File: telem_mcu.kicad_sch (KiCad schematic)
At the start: 28 parts, among them J3 Conn_01x06, J5 Micro_SD_Card, SW2 SW_Push, U3 STM32F373CCTx, X1 32.768kHz

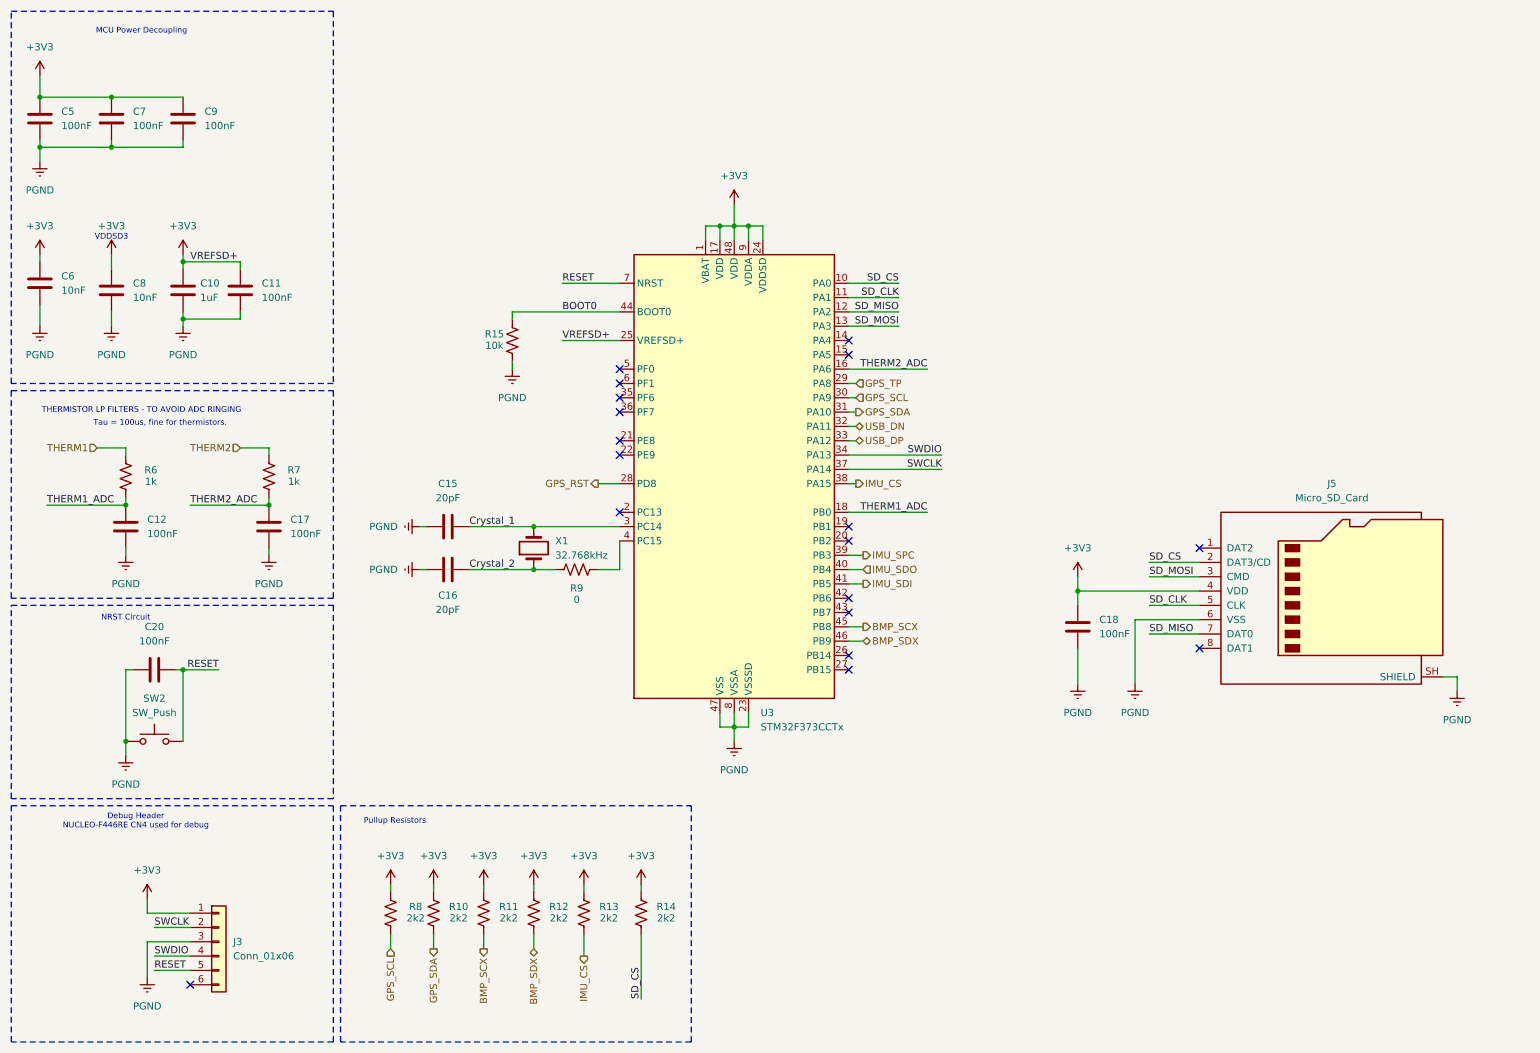
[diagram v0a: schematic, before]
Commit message: Updated schematics for rev2
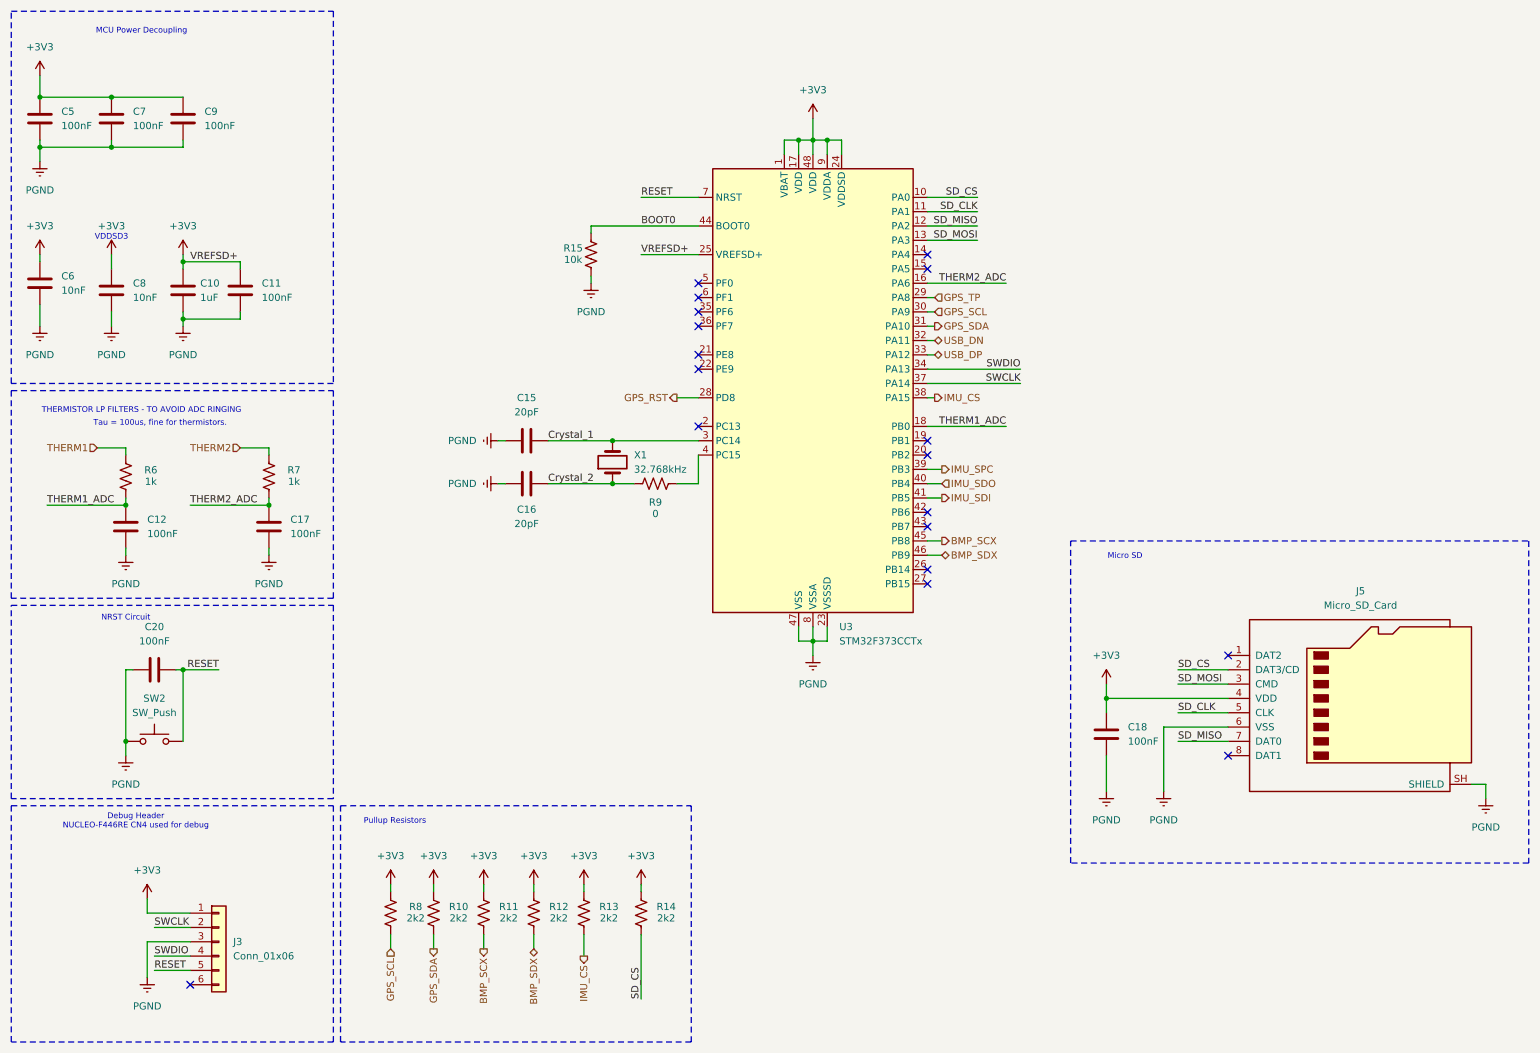
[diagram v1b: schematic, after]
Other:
- note added: "Micro SD"
- moved on the sheet: C15, C16, C18, J5, R15, R9, U3, X1
